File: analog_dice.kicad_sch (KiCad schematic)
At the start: 22 parts, among them SW1 SW_SPST, U1 LMC555xM, U2 4017

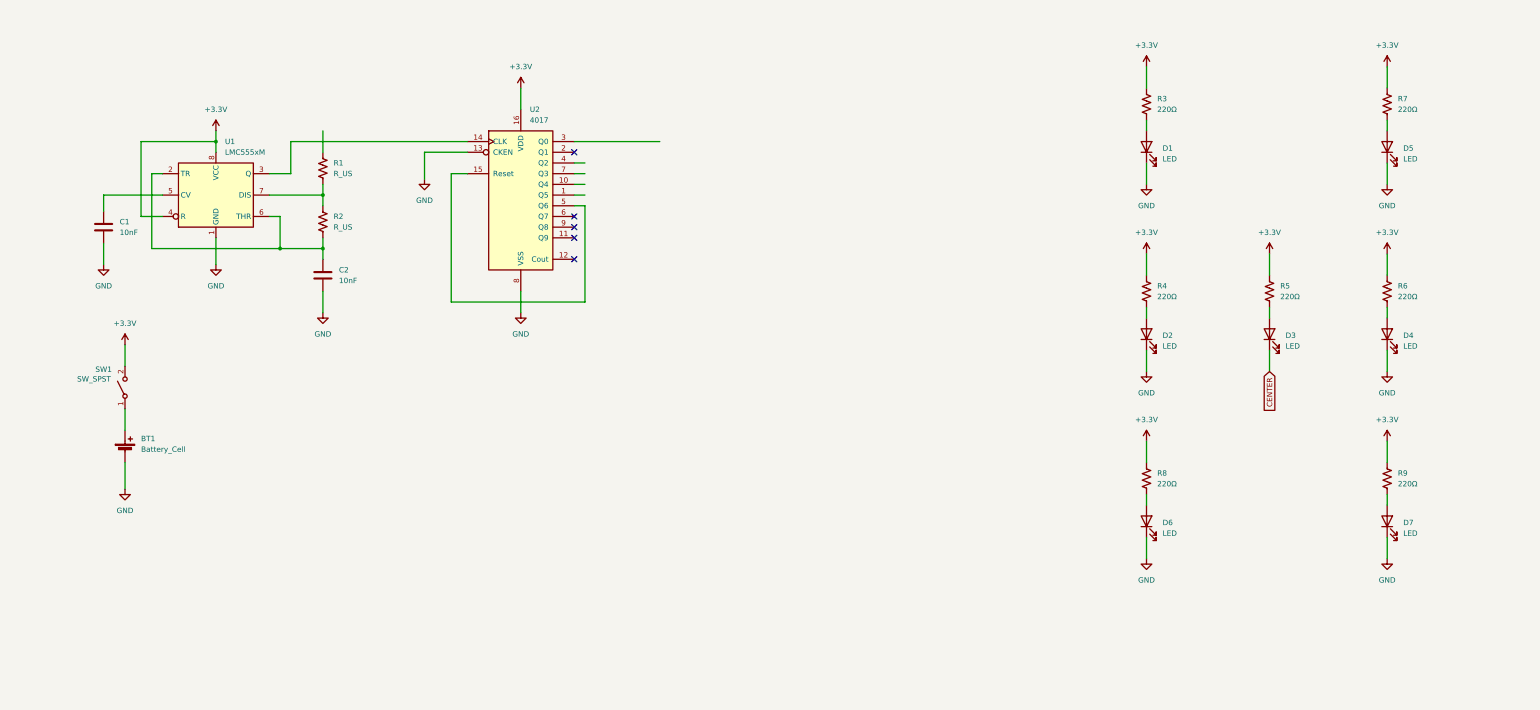
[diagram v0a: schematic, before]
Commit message: Update analog_dice.kicad_sch
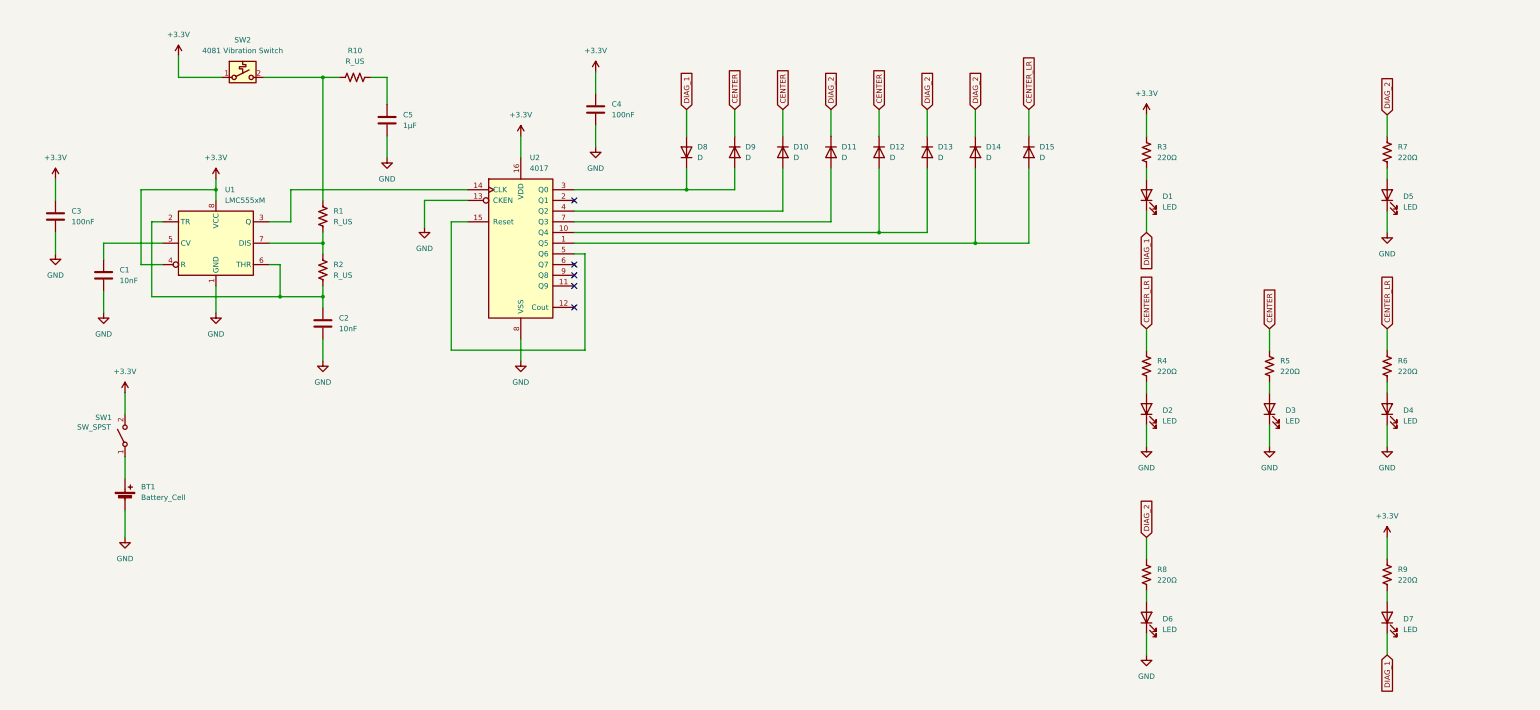
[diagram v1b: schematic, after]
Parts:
- added C3, C4: 100nF, symbol Device:C
- added C5: 1μF, symbol Device:C
- added D10, D11, D12, D13, D14, D15, D8, D9: D, symbol Device:D
- added R10: R_US, symbol Device:R_US
- added SW2: 4081 Vibration Switch, symbol Switch:SW_SPST_Temperature
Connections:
- net +3.3V: now also C3.1, C4.1, SW2.1 (A); no longer R4.1, R5.1, R6.1, R7.1, R8.1
- net CENTER: now also R5.1, D10.1 (K), D12.1 (K), D9.1 (K); no longer D3.1 (K)
- net GND: now also D3.1 (K), C3.2, C4.2, C5.2; no longer D1.1 (K), D7.1 (K)
- net at U2.1 (Q5): now also D14.2 (A), D15.2 (A)
- net at U2.10 (Q4): now also D12.2 (A), D13.2 (A)
- net at U2.3 (Q0): now also D8.1 (K), D9.2 (A)
- net at U2.4 (Q2): now also D10.2 (A)
- net at U2.7 (Q3): now also D11.2 (A)
- net at R1.1: now also R10.1, SW2.2 (B)
- new net: C5.1, R10.2
- new net CENTER_LR: D15.1 (K), R4.1, R6.1
- new net DIAG_1: D1.1 (K), D7.1 (K), D8.2 (A)
- new net DIAG_2: D11.1 (K), D13.1 (K), D14.1 (K), R7.1, R8.1
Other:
- moved on the sheet: BT1, C1, C2, D1, D2, D3, D4, D5, D6, D7, R1, R2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

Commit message: finish?
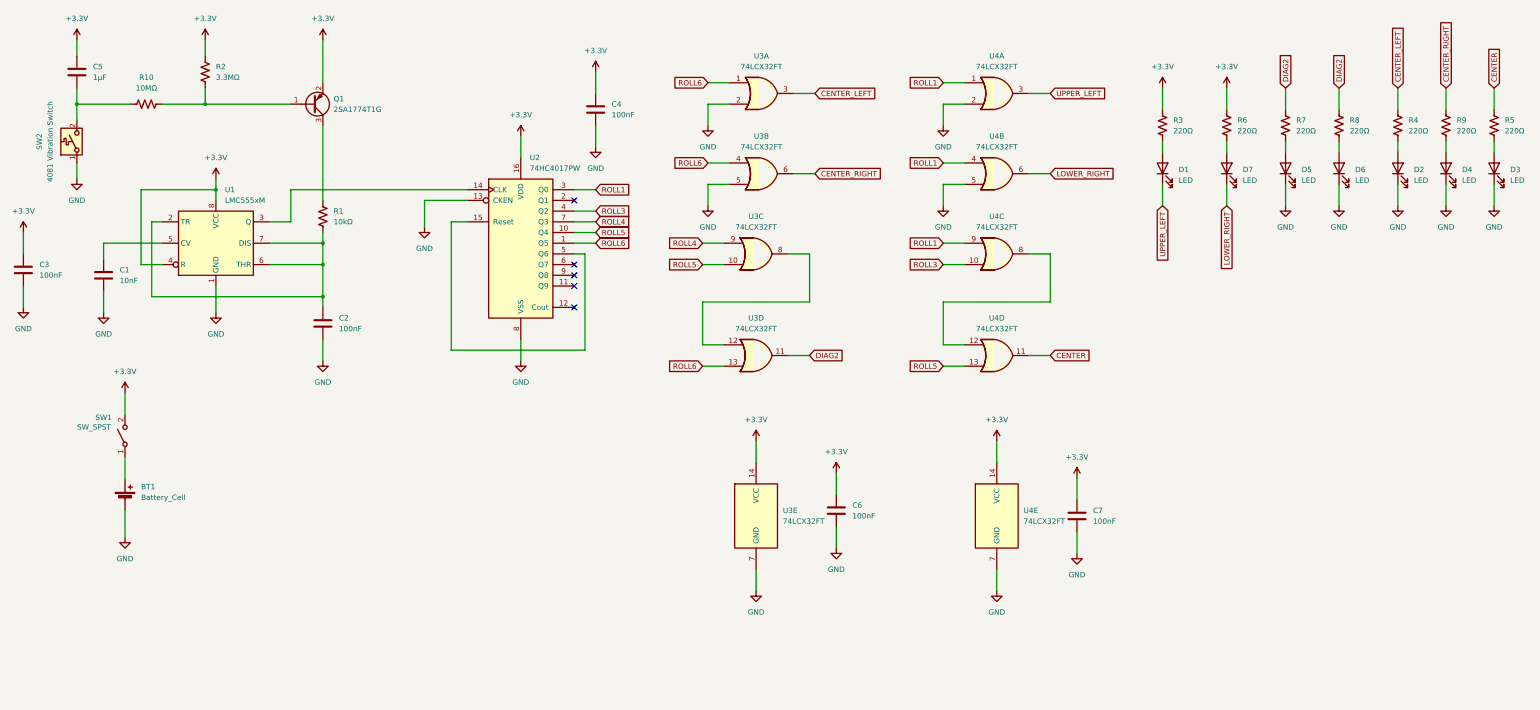
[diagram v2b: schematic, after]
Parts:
- removed D10, D11, D12, D13, D14, D15, D8, D9: D, symbol Device:D
- added C6, C7: 100nF, Capacitor_SMD:C_0201_0603Metric, symbol Device:C
- added Q1: 2SA1774T1G, Package_TO_SOT_SMD:SOT-416, symbol Transistor_BJT:Q_PNP_BEC
- added U3, U4: 74LCX32FT, Package_SO:TSSOP-14_4.4x5mm_P0.65mm, symbol 74xx:74LS32
- BT1: footprint (none) -> footprints:BAT-HLD-001; Manufacturer Part Number (none) -> BAT-HLD-001; Vendor (none) -> LCSC; Vendor Part Number (none) -> C7501066
- C1: footprint (none) -> Capacitor_SMD:C_0201_0603Metric; Manufacturer Part Number (none) -> GRM033R71A103KA01D; Vendor (none) -> LCSC; Vendor Part Number (none) -> C76941
- C2: value 10nF -> 100nF; footprint (none) -> Capacitor_SMD:C_0201_0603Metric; Manufacturer Part Number (none) -> GRM033R61A104KE15D; Vendor (none) -> LCSC; Vendor Part Number (none) -> C76934
- C3, C4: footprint (none) -> Capacitor_SMD:C_0201_0603Metric; Manufacturer Part Number (none) -> GRM033R61A104KE15D; Vendor (none) -> LCSC; Vendor Part Number (none) -> C76934
- C5: footprint (none) -> Capacitor_SMD:C_0201_0603Metric; Manufacturer Part Number (none) -> CL03A105MQ3CSNH; Vendor (none) -> LCSC; Vendor Part Number (none) -> C53067
- D1, D2, D3, D4, D5, D6, D7: footprint (none) -> LED_SMD:LED_0805_2012Metric; Manufacturer Part Number (none) -> YLED0805G; Vendor (none) -> LCSC; Vendor Part Number (none) -> C25170728
- R1: value R_US -> 10kΩ; footprint (none) -> Resistor_SMD:R_0201_0603Metric; Manufacturer Part Number (none) -> RC0201FR-0710KL; Vendor (none) -> LCSC; Vendor Part Number (none) -> C106225
- R10: value R_US -> 10MΩ; footprint (none) -> Resistor_SMD:R_0201_0603Metric; Manufacturer Part Number (none) -> 0201WMF1005TEE; Vendor (none) -> LCSC; Vendor Part Number (none) -> C423797
- R2: value R_US -> 3.3MΩ; footprint (none) -> Resistor_SMD:R_0201_0603Metric; Manufacturer Part Number (none) -> RK73B1HTTC335J; Vendor (none) -> LCSC; Vendor Part Number (none) -> C307099
- R3, R4, R5, R6, R7, R8, R9: footprint (none) -> Resistor_SMD:R_0201_0603Metric; Manufacturer Part Number (none) -> RC0201FR-07220RL; Vendor (none) -> LCSC; Vendor Part Number (none) -> C274342
- SW1: footprint (none) -> Button_Switch_SMD:SW_DIP_SPSTx01_Slide_Copal_CHS-01A_W5.08mm_P1.27mm_JPin; Manufacturer Part Number (none) -> CHS-01A1; Vendor (none) -> LCSC; Vendor Part Number (none) -> C3312106
- SW2: footprint (none) -> footprints:4081
- U1: Manufacturer Part Number (none) -> LMC555CMX/NOPB; Vendor (none) -> LCSC; Vendor Part Number (none) -> C90760
- U2: value 4017 -> 74HC4017PW; footprint (none) -> Package_SO:TSSOP-16_4.4x5mm_P0.65mm; Manufacturer Part Number (none) -> 74HC4017PW,118; Vendor (none) -> LCSC; Vendor Part Number (none) -> C546954
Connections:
- net +3.3V: now also C5.1, R2.2, R6.1, C6.1, C7.1, Q1.2 (E), U3.14 (VCC), U4.14 (VCC); no longer R9.1, SW2.1 (A)
- net CENTER: now also U4.11
- net GND: now also SW2.1 (A), C6.2, C7.2, U3.2, U3.5, U3.7 (GND), U4.2, U4.5, U4.7 (GND); no longer C5.2
- net ROLL1: now reaches U2.3 (Q0)
- net ROLL1: now also U4.1, U4.4, U4.9
- net ROLL5: now reaches U2.10 (Q4)
- net ROLL5: now also U3.10, U4.13
- net ROLL4: now reaches U2.7 (Q3)
- net ROLL4: now also U3.9
- net at R6.2: now also D7.2 (A); no longer D4.2 (A)
- net at C2.1, U1.2 (TR), U1.6 (THR): now also R1.2, U1.7 (DIS); no longer R2.2
- net ROLL3: now reaches U2.4 (Q2)
- net ROLL3: now also U4.10
- net at R10.1, SW2.2 (B): now also C5.2; no longer R1.1
- net at R10.2: now also R2.1, Q1.1 (B); no longer C5.1
- net ROLL6: now reaches U2.1 (Q5)
- net ROLL6: now also U3.1, U3.13, U3.4
- net at R9.2: now also D4.2 (A); no longer D7.2 (A)
- net CENTER_LR renamed CENTER_LEFT
- net CENTER_LEFT: now also U3.3; no longer R6.1
- net DIAG_1 renamed LOWER_RIGHT
- net LOWER_RIGHT: now also U4.6; no longer D1.1 (K)
- net DIAG_2 renamed DIAG2
- net DIAG2: now also U3.11
- new net: U3.12, U3.8
- new net: Q1.3 (C), R1.1
- new net: U4.12, U4.8
- new net CENTER_RIGHT: R9.1, U3.6
- new net UPPER_LEFT: D1.1 (K), U4.3
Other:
- moved on the sheet: C3, C5, D1, D2, D3, D4, D5, D6, D7, R10, R3, R4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
